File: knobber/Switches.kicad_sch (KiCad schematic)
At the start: 24 parts, among them SW101 SW_Push, SW102 SW_Push, SW103 SW_Push, SW104 SW_Push, SW105 SW_Push, SW701 SW_Push

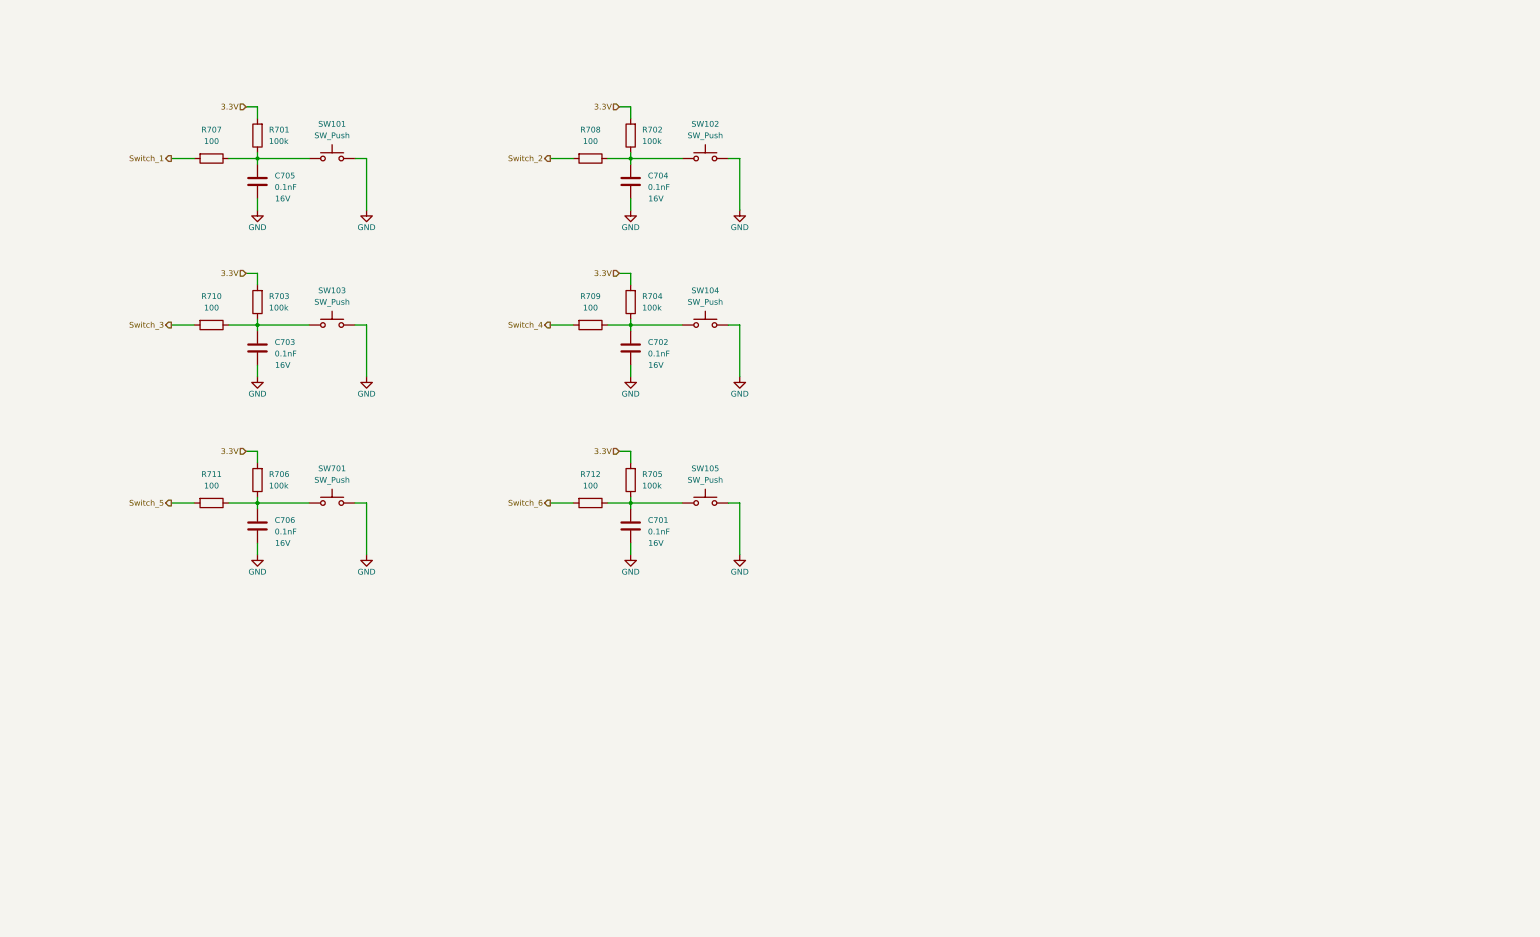
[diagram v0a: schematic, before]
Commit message: updated schematic
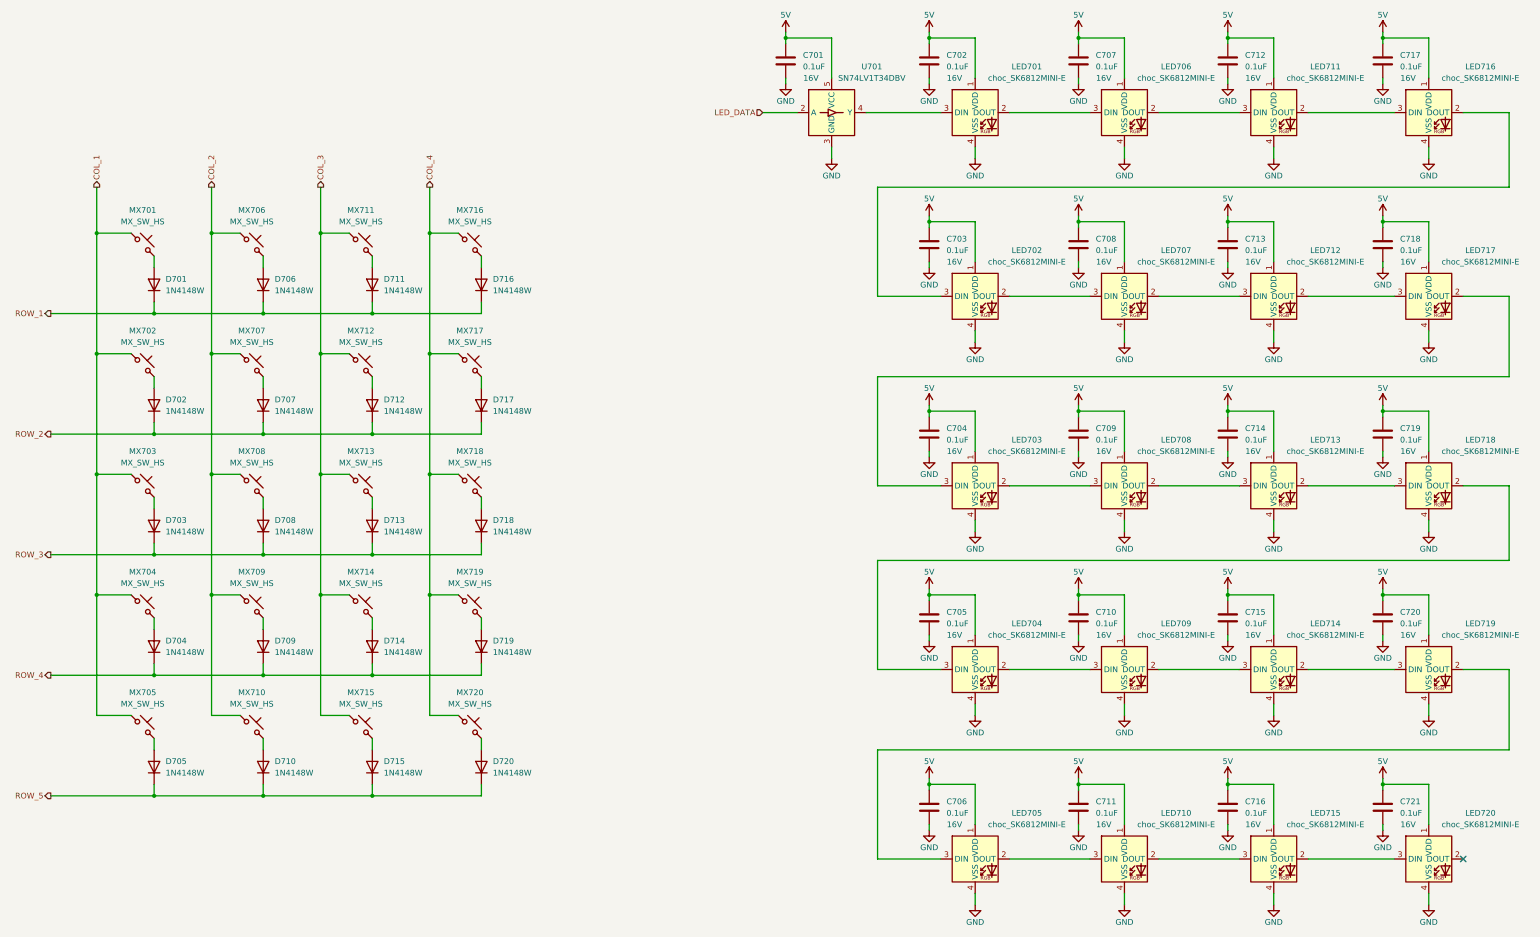
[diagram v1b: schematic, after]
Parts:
- removed R701, R702, R703, R704, R705, R706: 100k, Resistor_SMD:R_0603_1608Metric, symbol Device:R
- removed R707, R708, R709, R710, R711, R712: 100, Resistor_SMD:R_0603_1608Metric, symbol Device:R
- removed SW101, SW102, SW103, SW104, SW105, SW701: SW_Push, PCM_Switch_Keyboard_Hotswap_Kailh:SW_Hotswap_Kailh_Choc_V1V2_1.00u, symbol Switch:SW_Push
- added C707, C708, C709, C710, C711, C712, C713, C714, C715, C716, C717, C718, C719, C720, C721: 0.1uF, Capacitor_SMD:C_0603_1608Metric, symbol Device:C
- added D701, D702, D703, D704, D705, D706, D707, D708, D709, D710, D711, D712, D713, D714, D715, D716, D717, D718, D719, D720: 1N4148W, Diode_SMD:D_SOD-123, symbol Diode:1N4148W
- added LED701, LED702, LED703, LED704, LED705, LED706, LED707, LED708, LED709, LED710, LED711, LED712, LED713, LED714, LED715, LED716, LED717, LED718, LED719, LED720: choc_SK6812MINI-E, PCM_marbastlib-choc:LED_choc_6028R, symbol PCM_marbastlib-choc:choc_SK6812MINI-E
- added MX701, MX702, MX703, MX704, MX705, MX706, MX707, MX708, MX709, MX710, MX711, MX712, MX713, MX714, MX715, MX716, MX717, MX718, MX719, MX720: MX_SW_HS, PCM_marbastlib-mx:SW_MX_HS_CPG151101S11_1u, symbol PCM_marbastlib-mx:MX_SW_HS_CPG151101S11
- added U701: SN74LV1T34DBV, Package_TO_SOT_SMD:SOT-23-5, symbol Logic_LevelTranslator:SN74LV1T34DBV
- C701, C702, C703, C704, C705, C706: value 0.1nF -> 0.1uF; footprint Capacitor_SMD:C_0805_2012Metric -> Capacitor_SMD:C_0603_1608Metric
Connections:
- net GND: now also C707.2, C708.2, C709.2, C710.2, C711.2, C712.2, C713.2, C714.2, C715.2, C716.2, C717.2, C718.2, C719.2, C720.2, C721.2, LED701.4 (VSS), LED702.4 (VSS), LED703.4 (VSS), LED704.4 (VSS), LED705.4 (VSS), LED706.4 (VSS), LED707.4 (VSS), LED708.4 (VSS), LED709.4 (VSS), LED710.4 (VSS), LED711.4 (VSS), LED712.4 (VSS), LED713.4 (VSS), LED714.4 (VSS), LED715.4 (VSS), LED716.4 (VSS), LED717.4 (VSS), LED718.4 (VSS), LED719.4 (VSS), LED720.4 (VSS), U701.3 (GND)
- net 5V: now reaches C703.1
- net 5V: now also C701.1, C702.1, C704.1, C705.1, C706.1, C707.1, C708.1, C709.1, C710.1, C711.1, C712.1, C713.1, C714.1, C715.1, C716.1, C717.1, C718.1, C719.1, C720.1, C721.1, LED701.1 (VDD), LED702.1 (VDD), LED703.1 (VDD), LED704.1 (VDD), LED705.1 (VDD), LED706.1 (VDD), LED707.1 (VDD), LED708.1 (VDD), LED709.1 (VDD), LED710.1 (VDD), LED711.1 (VDD), LED712.1 (VDD), LED713.1 (VDD), LED714.1 (VDD), LED715.1 (VDD), LED716.1 (VDD), LED717.1 (VDD), LED718.1 (VDD), LED719.1 (VDD), LED720.1 (VDD), U701.5 (VCC)
- new net: LED703.3 (DIN), LED717.2 (DOUT)
- new net: LED712.2 (DOUT), LED717.3 (DIN)
- new net: D710.2 (A), MX710.2
- new net: LED705.2 (DOUT), LED710.3 (DIN)
- new net: LED705.3 (DIN), LED719.2 (DOUT)
- new net: D709.2 (A), MX709.2
- new net: LED706.2 (DOUT), LED711.3 (DIN)
- new net: LED701.2 (DOUT), LED706.3 (DIN)
- new net: LED702.2 (DOUT), LED707.3 (DIN)
- new net: LED702.3 (DIN), LED716.2 (DOUT)
- new net: D717.2 (A), MX717.2
- new net: D716.2 (A), MX716.2
- new net: D707.2 (A), MX707.2
- new net: LED711.2 (DOUT), LED716.3 (DIN)
- new net: D719.2 (A), MX719.2
- new net: D711.2 (A), MX711.2
- new net: LED709.2 (DOUT), LED714.3 (DIN)
- new net: LED704.2 (DOUT), LED709.3 (DIN)
- new net: LED714.2 (DOUT), LED719.3 (DIN)
- new net: D720.2 (A), MX720.2
- new net: D712.2 (A), MX712.2
- new net: LED707.2 (DOUT), LED712.3 (DIN)
- new net: D708.2 (A), MX708.2
- new net: D715.2 (A), MX715.2
- new net: LED701.3 (DIN), U701.4 (Y)
- new net: D705.2 (A), MX705.2
- new net: D704.2 (A), MX704.2
- new net: LED703.2 (DOUT), LED708.3 (DIN)
- new net: LED713.2 (DOUT), LED718.3 (DIN)
- new net: LED708.2 (DOUT), LED713.3 (DIN)
- new net: LED715.2 (DOUT), LED720.3 (DIN)
- new net: LED710.2 (DOUT), LED715.3 (DIN)
- new net: LED704.3 (DIN), LED718.2 (DOUT)
- new net: D718.2 (A), MX718.2
- new net: D702.2 (A), MX702.2
- new net: D706.2 (A), MX706.2
- new net: D701.2 (A), MX701.2
- new net: D703.2 (A), MX703.2
- new net: D714.2 (A), MX714.2
- new net: D713.2 (A), MX713.2
- new net COL_1: MX701.1, MX702.1, MX703.1, MX704.1, MX705.1
- new net COL_2: MX706.1, MX707.1, MX708.1, MX709.1, MX710.1
- new net COL_3: MX711.1, MX712.1, MX713.1, MX714.1, MX715.1
- new net COL_4: MX716.1, MX717.1, MX718.1, MX719.1, MX720.1
- new net LED_DATA: U701.2 (A)
- new net ROW_1: D701.1 (K), D706.1 (K), D711.1 (K), D716.1 (K)
- new net ROW_2: D702.1 (K), D707.1 (K), D712.1 (K), D717.1 (K)
- new net ROW_3: D703.1 (K), D708.1 (K), D713.1 (K), D718.1 (K)
- new net ROW_4: D704.1 (K), D709.1 (K), D714.1 (K), D719.1 (K)
- new net ROW_5: D705.1 (K), D710.1 (K), D715.1 (K), D720.1 (K)
- no-connect marks 0 -> 1
